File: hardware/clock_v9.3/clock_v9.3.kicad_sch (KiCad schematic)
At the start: 114 parts, among them J1 Conn_01x06, J2 Conn_01x10, J3 Conn_01x10, J4 USB_C_Receptacle, J8 Conn_01x02, U1 SN74LVC1G14DBV, U11 AMS1117-3.3, U12 BA50DD0WHFP-TR, U14 CH340C, U15 USBLC6-2P6, U2 SN74LVC1G14DBV, U23 TPS63060, U3 SN74LVC1G14DBV, U4 LM2731XMF, U5 LM2731XMF, U9 L78L05_SOT89

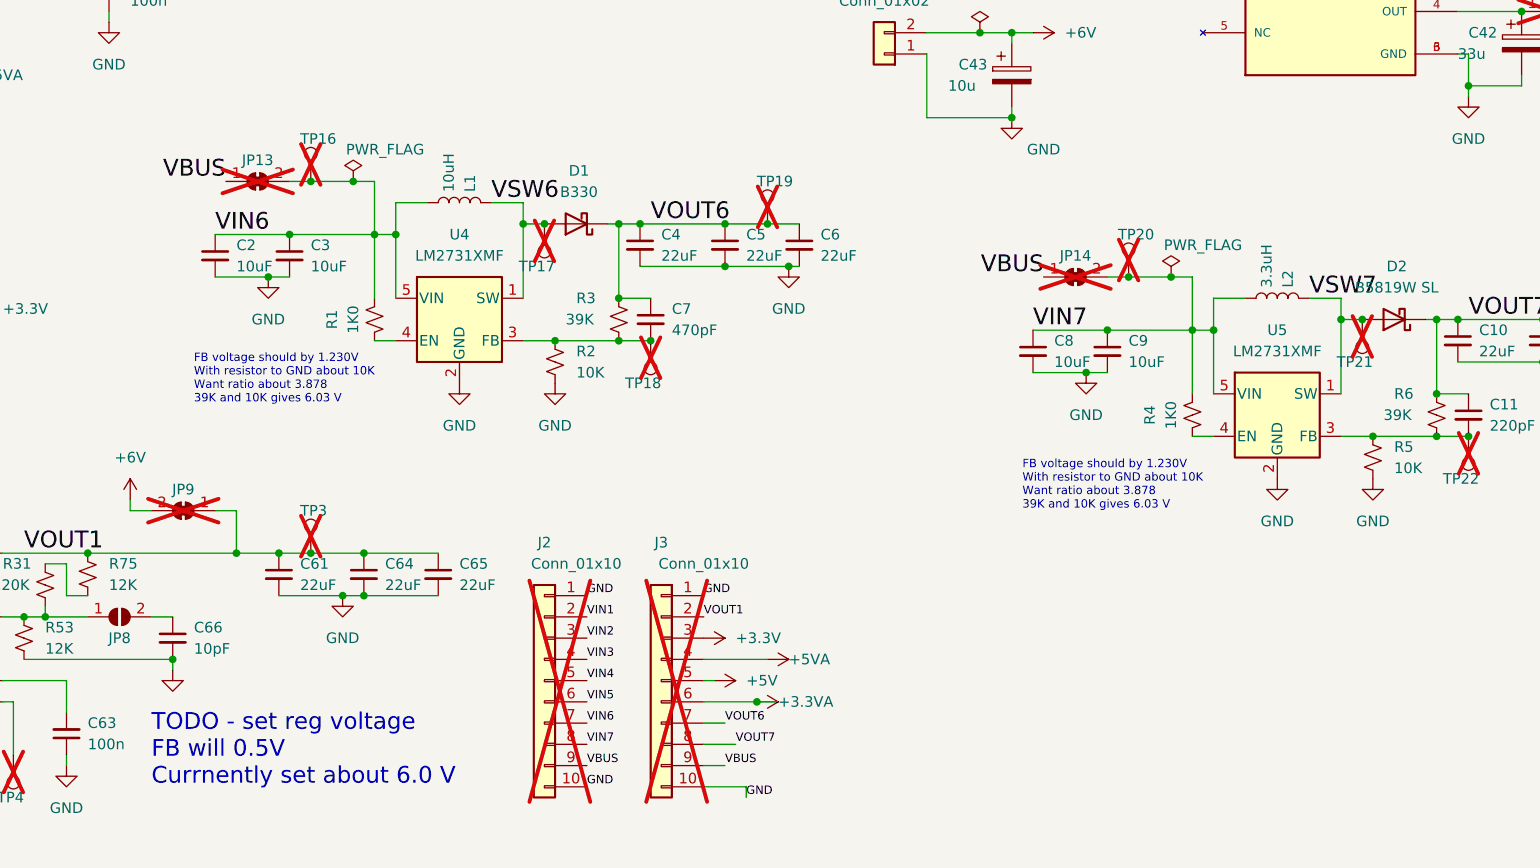
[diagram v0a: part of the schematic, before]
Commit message: clean up
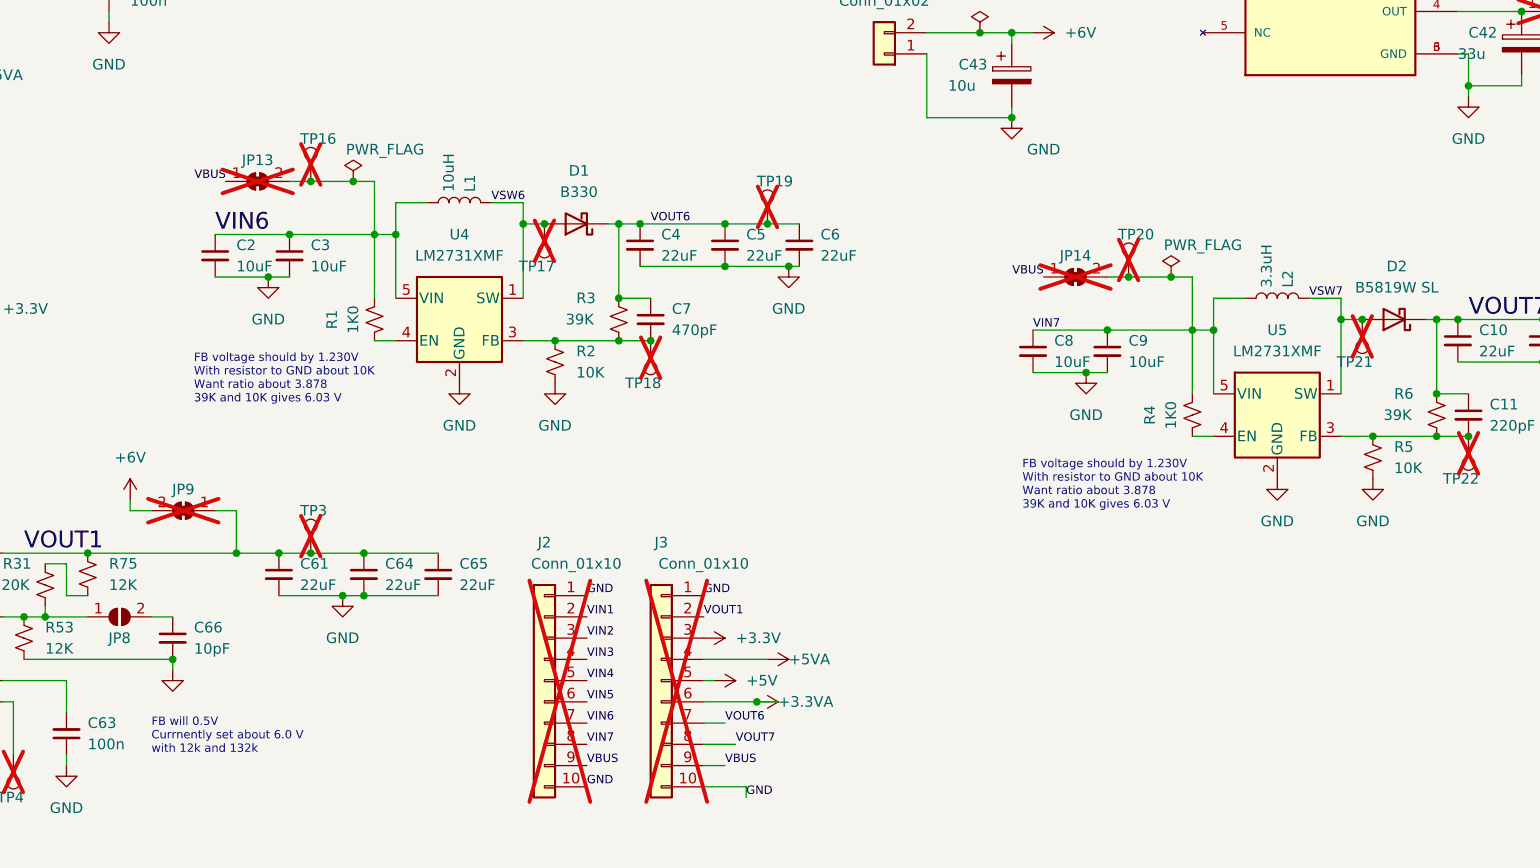
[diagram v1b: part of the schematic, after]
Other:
- note added: "FB will 0.5V Currnently set about 6.0 V with 12k and 132k"
- note removed: "TODO - set reg voltage FB will 0.5V Currnently set about 6.0 V"
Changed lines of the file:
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@@
     (effects (font (size 1 1)) (justify left bottom))
   )
-  (text "TODO - set reg voltage\nFB will 0.5V \nCurrnently set about 6.0 V "
-    (at 93.98 187.96 0)
-    (effects (font (size 2 2)) (justify left bottom))
+  (text "FB will 0.5V \nCurrnently set about 6.0 V \nwith 12k and 132k "
+    (at 93.98 184.15 0)
+    (effects (font (size 1 1)) (justify left bottom))
   )
   (text "FB voltage should by 1.230V \nWith resistor to GND about 10K \nWant ratio about 3.878\n39K and 10K gives 6.03 V\n"
@@
   )
   (label "VOUT6" (at 153.67 120.65 0) (fields_autoplaced)
-    (effects (font (size 2 2)) (justify left bottom))
+    (effects (font (size 1 1)) (justify left bottom))
   )
   (label "GND" (at 146.05 187.96 0) (fields_autoplaced)
@@
   )
   (label "VSW7" (at 232.41 129.54 0) (fields_autoplaced)
-    (effects (font (size 2 2)) (justify left bottom))
+    (effects (font (size 1 1)) (justify left bottom))
   )
   (label "BOOT0" (at 114.3 34.29 0) (fields_autoplaced)
@@
   )
   (label "VSW6" (at 134.62 118.11 0) (fields_autoplaced)
-    (effects (font (size 2 2)) (justify left bottom))
+    (effects (font (size 1 1)) (justify left bottom))
   )
   (label "NRST" (at 120.65 55.88 0) (fields_autoplaced)
@@
   )
   (label "VIN7" (at 199.39 133.35 0) (fields_autoplaced)
-    (effects (font (size 2 2)) (justify left bottom))
+    (effects (font (size 1 1)) (justify left bottom))
   )
   (label "VIN3" (at 146.05 172.72 0) (fields_autoplaced)
@@
   )
   (label "VBUS" (at 200.66 127 180) (fields_autoplaced)
-    (effects (font (size 2 2)) (justify right bottom))
+    (effects (font (size 1 1)) (justify right bottom))
   )
   (label "VIN5" (at 146.05 177.8 0) (fields_autoplaced)
@@
   )
   (label "VBUS" (at 102.87 115.57 180) (fields_autoplaced)
-    (effects (font (size 2 2)) (justify right bottom))
+    (effects (font (size 1 1)) (justify right bottom))
   )
   (label "VIN1" (at 55.88 160.02 180) (fields_autoplaced)
